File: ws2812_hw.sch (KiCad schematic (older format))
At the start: 6 parts

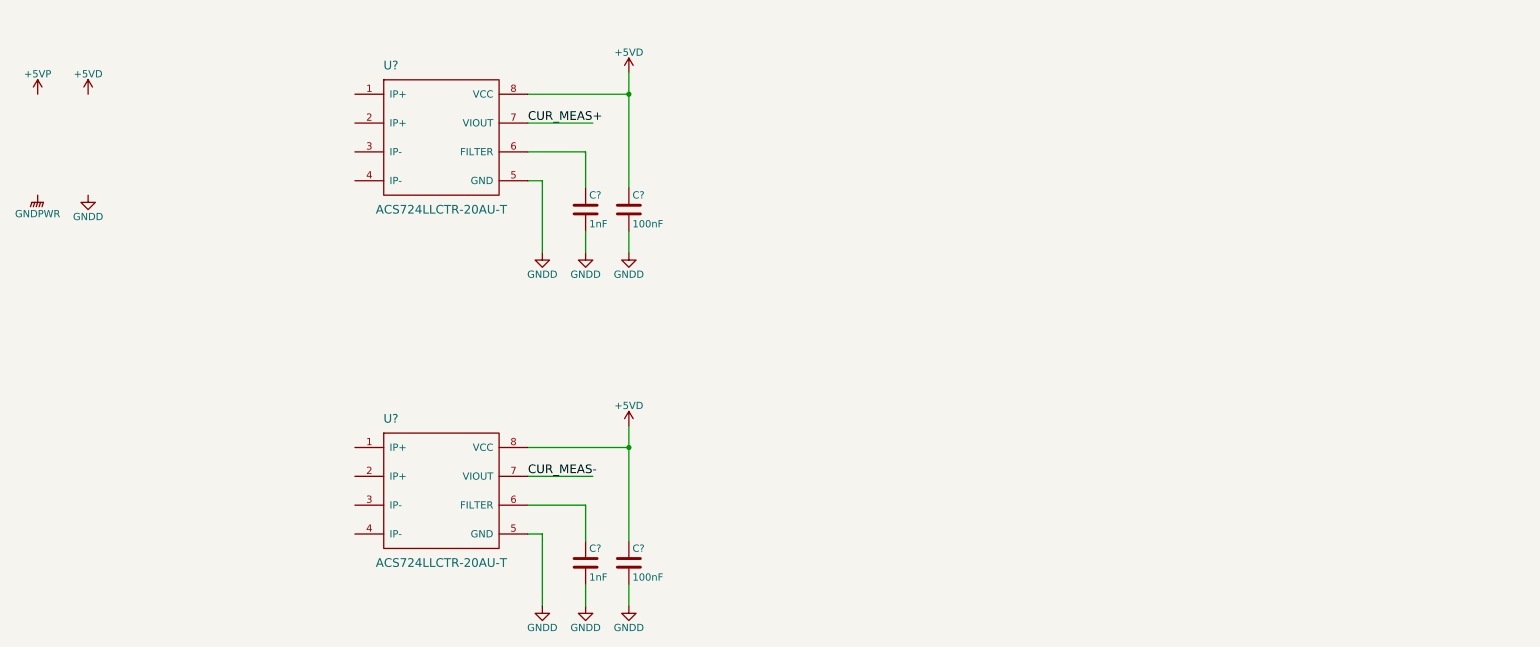
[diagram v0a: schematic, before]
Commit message: further work
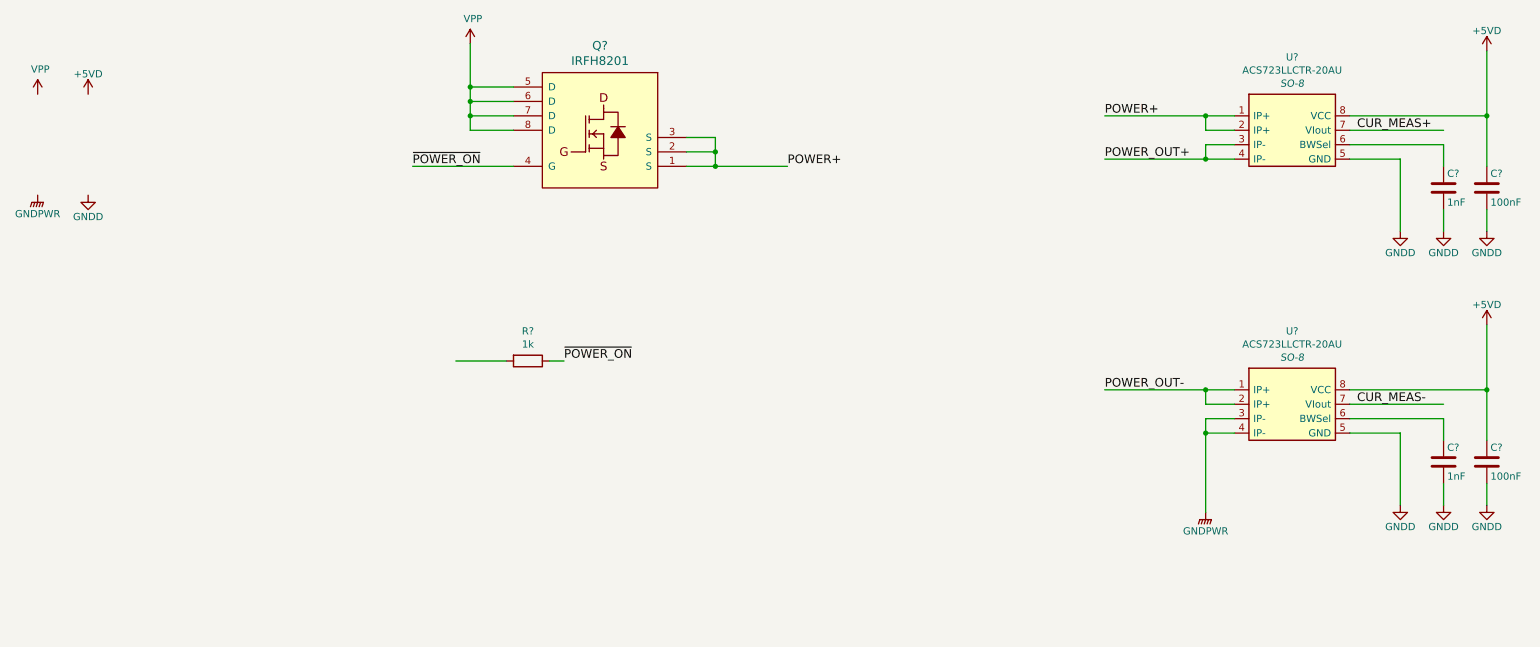
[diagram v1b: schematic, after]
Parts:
- removed C?: 1nF, symbol C
- removed C?: 100nF, symbol C
- removed U? (x2): ACS724LLCTR-20AU-T, symbol ACS724
- added C?: 1nF, symbol C
- added C?: 100nF, symbol C
- added Q?: IRFH8201, symbol IRFH8201-RESCUE-ws2812_hw
- added R?: 1k, symbol R
- added U? (x2): ACS723LLCTR-20AU, SO-8, symbol ACS723LLCTR-20AU
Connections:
- net labels added: POWER+, POWER_OUT+, POWER_OUT-, VPP, ~POWER_ON
- net labels removed: +5VP
- wire segments 18 -> 42
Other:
- moved on the sheet: C?
